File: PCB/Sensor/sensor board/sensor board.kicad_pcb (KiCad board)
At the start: 2 copper layers, 39.2 x 71.9 mm, 28 parts, among them J1 Conn_01x07, J2 JST-XH, J3 INPUT, SW1 SW_Push, SW2 SW_Push, U1 ESP32-S3-WROOM-1-N16R2

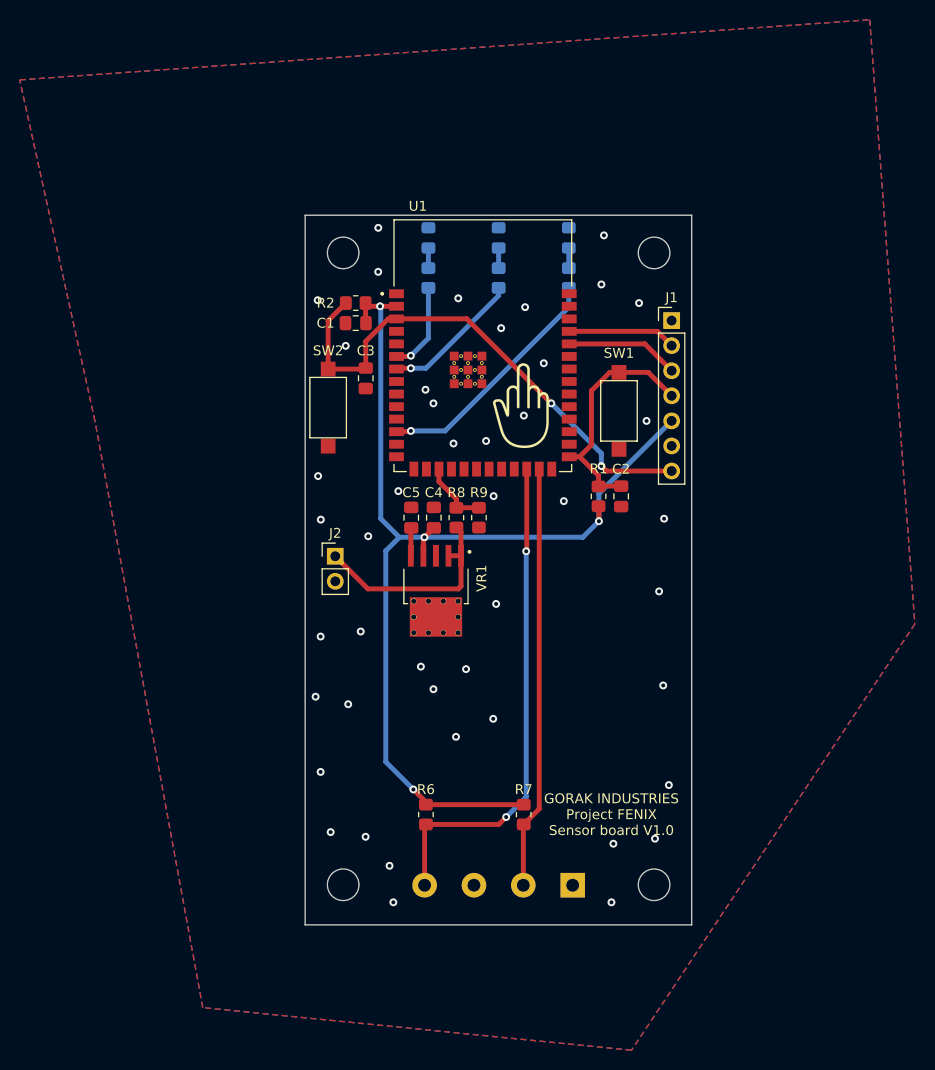
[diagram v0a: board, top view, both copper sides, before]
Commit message: sensor V1.1 + gerbery
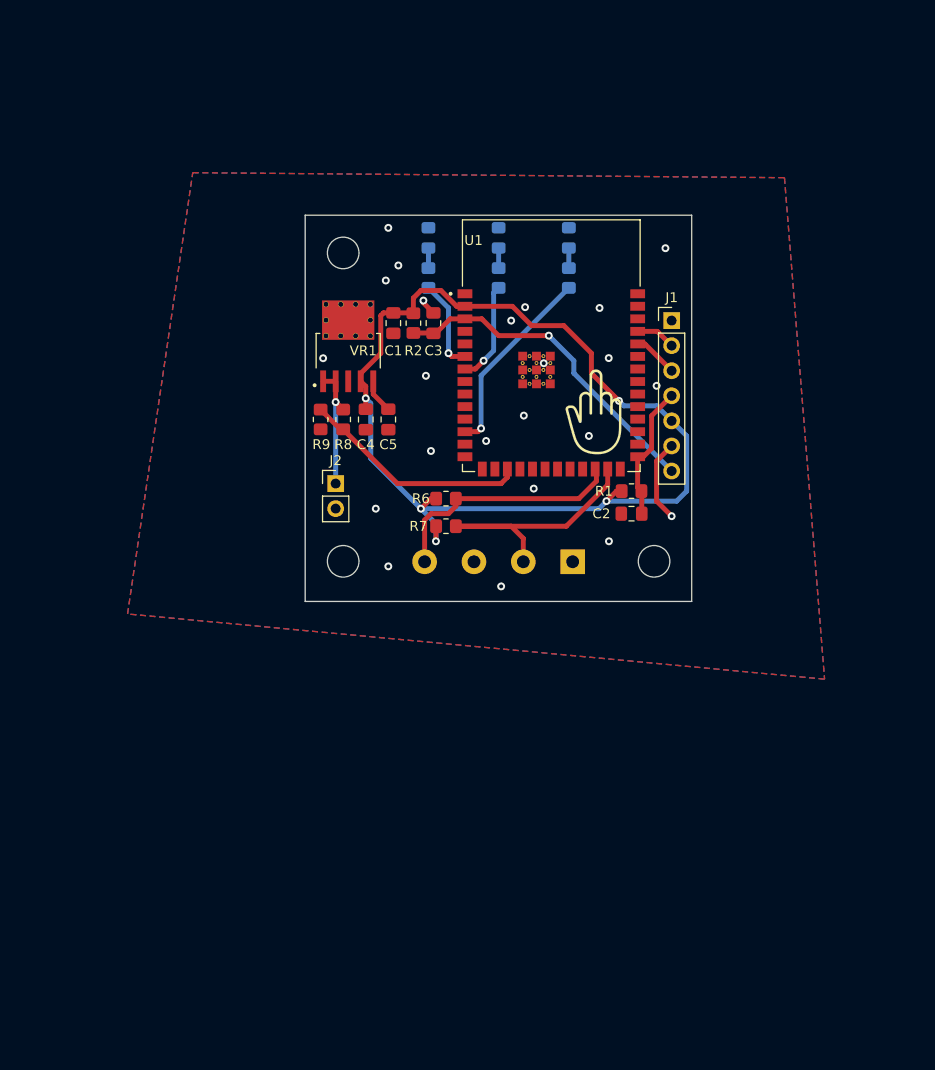
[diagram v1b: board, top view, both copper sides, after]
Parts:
- removed the REF** at (117.3, 84.3)
- removed SW1, SW2: SW_Push, Button_Switch_SMD:SW_SPST_CK_RS282G05A3
- moved REF** 32.8 mm to (85.9, 115.6)
- moved REF** 32.8 mm to (117.3, 115.6)
- moved J3 32.8 mm to (109.1, 115.6)
- moved R6 32.1 mm to (96.3, 109.2), turned to 0 degrees
- moved R7 30.3 mm to (96.3, 112.0), turned to 0 degrees
- moved VR1 25.5 mm to (86.4, 94.2), turned to 90 degrees
- moved R9 18.9 mm to (83.6, 101.2)
- moved R8 15.2 mm to (85.9, 101.2), turned to -90 degrees
- moved C4 12.1 mm to (88.1, 101.2), turned to -90 degrees
- moved C5 10.2 mm to (90.4, 101.2), turned to -90 degrees
- moved C3 8.85 mm to (95.0, 91.4), turned to 90 degrees
- moved J2 7.37 mm to (85.1, 107.7)
- moved U1 6.93 mm to (106.9, 93.7)
- moved R2 6.19 mm to (93.0, 91.4), turned to -90 degrees
- moved C1 3.81 mm to (90.9, 91.4), turned to -90 degrees
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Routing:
- net S1: track 50.8 -> 25.0 mm, vias 2 -> 0
- net EN: track 53.1 -> 33.9 mm, vias 2 -> 1
- net BATT: track 6.93 -> 23.1 mm
- net S2: track 42.8 -> 28.4 mm
- net IO0: track 24.2 -> 13.9 mm
- net GND: track 0.00 -> 10.0 mm, vias 45 -> 23
- net VIN: track 21.6 -> 12.7 mm, vias 0 -> 1
- net TX0: track 11.0 -> 4.04 mm
- net RX0: track 11.5 -> 4.57 mm
- net LED1: track 24.6 -> 19.7 mm
- net LED2: track 14.2 -> 10.3 mm
- net +3.3V: track 107.7 -> 106.9 mm, vias 4 -> 5
- net Net-(C5-Pad1): track 2.84 -> 3.46 mm
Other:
- board size 39.2 x 71.9 mm -> 39.2 x 39.1 mm
- board text added: "GORAK INDUSTRIES Project FENIX Sensor board V1.1"
- board text removed: "GORAK INDUSTRIES Project FENIX Sensor board V1.0"
